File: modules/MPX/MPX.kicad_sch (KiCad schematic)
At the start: 26 parts, among them J1 SERIALA, J3 Conn_02x10_Odd_Even, SW1 PAGE SELECT, U1 W65C02, U10 74AHCT541, U12 74HC138, U14 74HC688, U15 74HC20, U16 74AHCT541, U2 CY62256-70PC, U3 28C256, U4 W65C22, U5 W65C51, U6 MAX232, U7 74AHCT541, U8 74AHCT541, U9 74AHCT245, Y2 1.8432Mhz

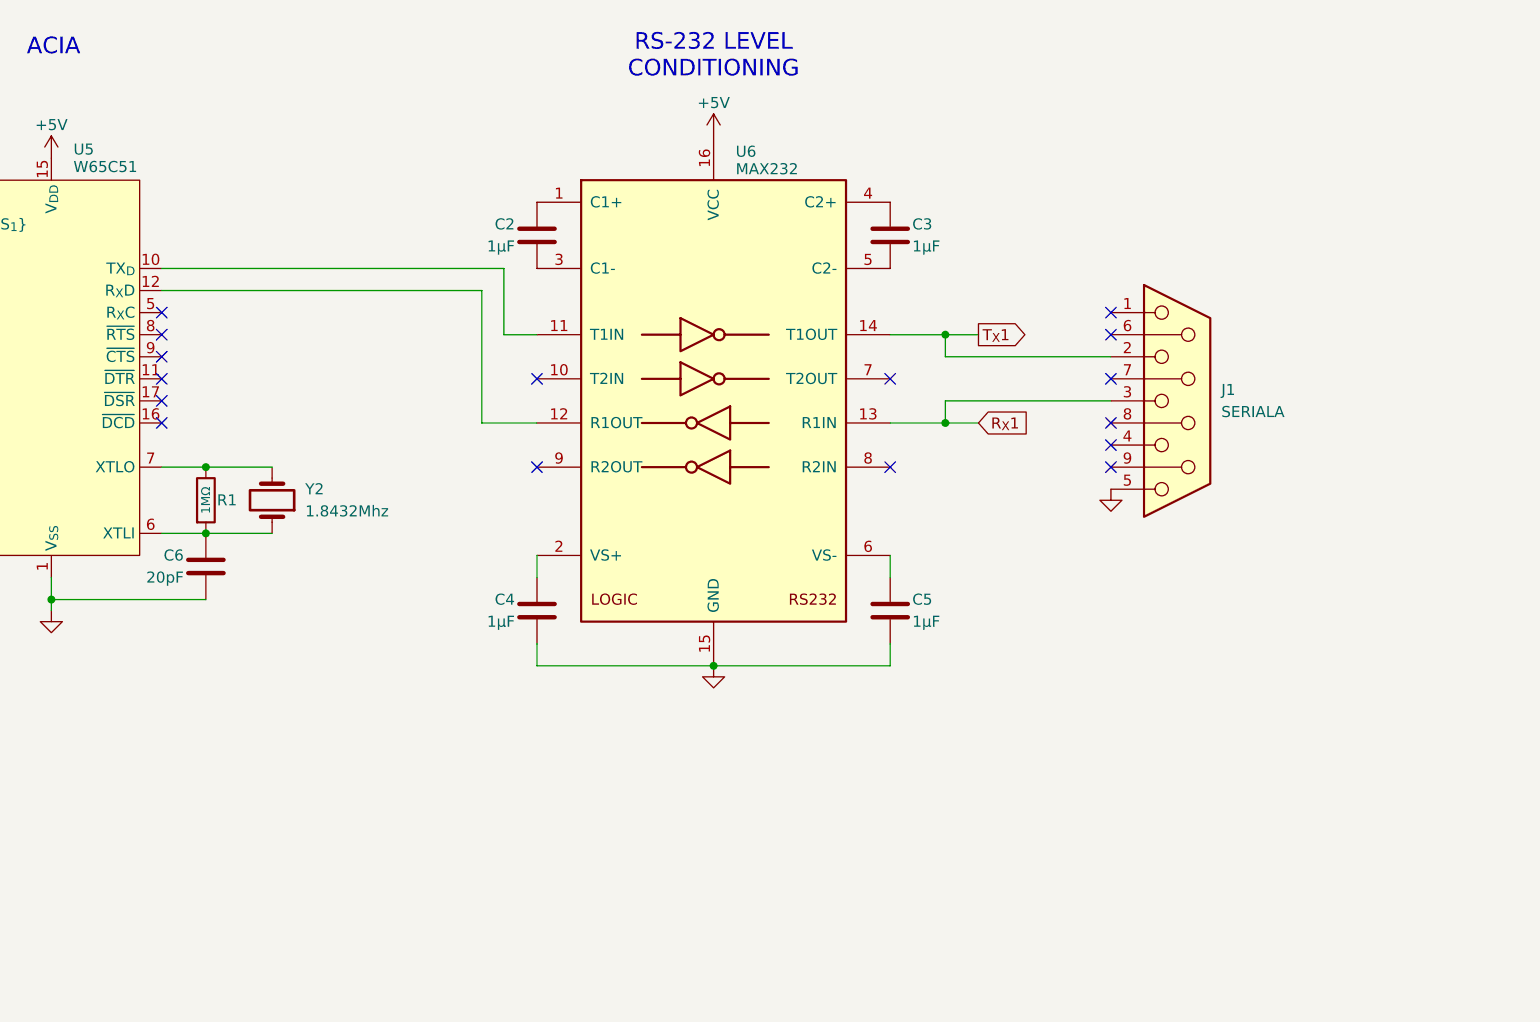
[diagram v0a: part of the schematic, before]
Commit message: sync
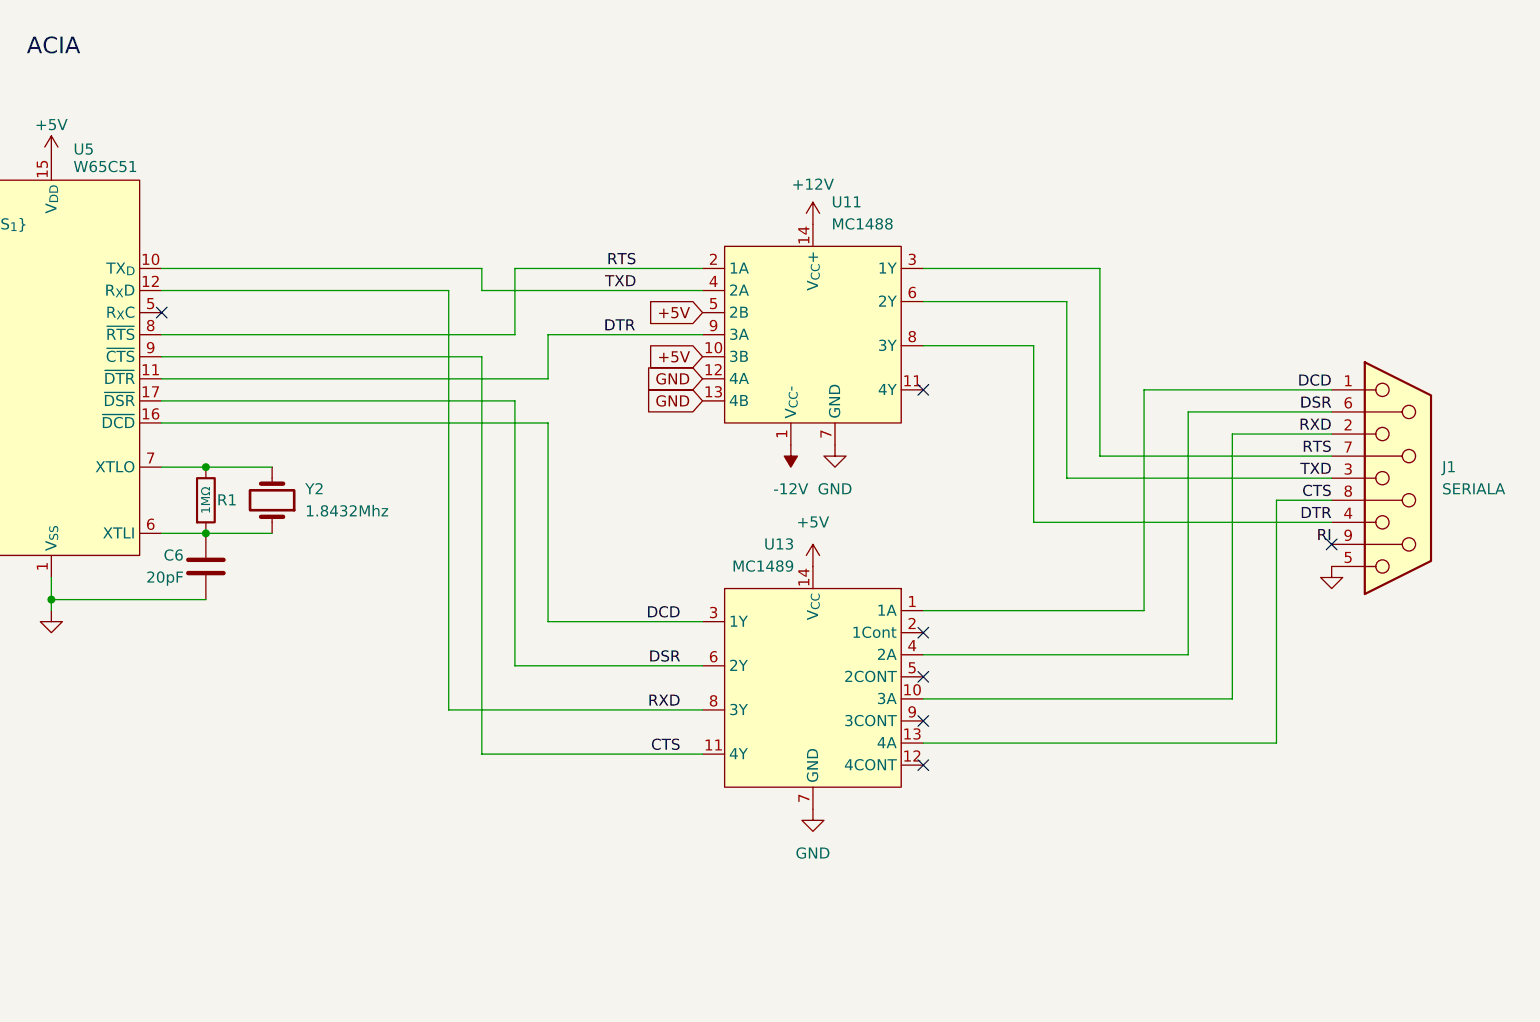
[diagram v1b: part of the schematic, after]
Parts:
- removed C2, C3, C4, C5: 1µF, IMNOTWOPR:C_Rect_P200mil, symbol IMNOTWOPR:C
- removed U6: MAX232, IMNOTWOPR:DIP-16N, symbol IMNOTWOPR:MAX232
- added U11: MC1488, IMNOTWOPR:DIP-14N, symbol IMNOTWOPR:MC1488
- added U13: MC1489, IMNOTWOPR:DIP-14N, symbol IMNOTWOPR:MC1489
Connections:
- net R_{X}1 is gone; now on net TXD: J1.3
- net T_{X}1 is gone; now on net RXD: J1.2
- net +5V: now also U11.10 (3B), U11.5 (2B), U13.14 (V_{CC})
- net GND: now also U11.12 (4A), U11.13 (4B), U11.7 (GND), U13.7 (GND)
- net DCD: now reaches J1.1
- net DCD: now also U5.16 (~{DCD}), U13.1 (1A), U13.3 (1Y)
- net DTR: now reaches J1.4
- net DTR: now also U5.11 (~{DTR}), U11.8 (3Y), U11.9 (3A)
- net DSR: now reaches J1.6
- net DSR: now also U5.17 (~{DSR}), U13.4 (2A), U13.6 (2Y)
- net RTS: now reaches J1.7
- net RTS: now also U5.8 (~{RTS}), U11.2 (1A), U11.3 (1Y)
- net CTS: now reaches J1.8
- net CTS: now also U5.9 (~{CTS}), U13.11 (4Y), U13.13 (4A)
- net RI: now reaches J1.9
- net TXD: now reaches U5.10 (TX_{D})
- net TXD: now also U11.4 (2A), U11.6 (2Y)
- net RXD: now reaches U5.12 (R_{X}D)
- net RXD: now also U13.10 (3A), U13.8 (3Y)
- new net +12V: U11.14 (V_{CC}+)
- new net -12V: U11.1 (V_{CC}-)
- no-connect marks 24 -> 15
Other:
- note removed: "RS-232 LEVEL CONDITIONING"
- moved on the sheet: J1
